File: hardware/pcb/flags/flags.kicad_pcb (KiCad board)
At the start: 2 copper layers, 62.2 x 21.6 mm, 42 parts, among them J1 Bus, J2 Control, J3 Sync, J4 Power, J5 Flags_Bus, J6 Ctrl_Out, U1 74HC02, U2 74HC08, U3 74HC157, U4 74HC173, U5 74HC173, U6 74HC125

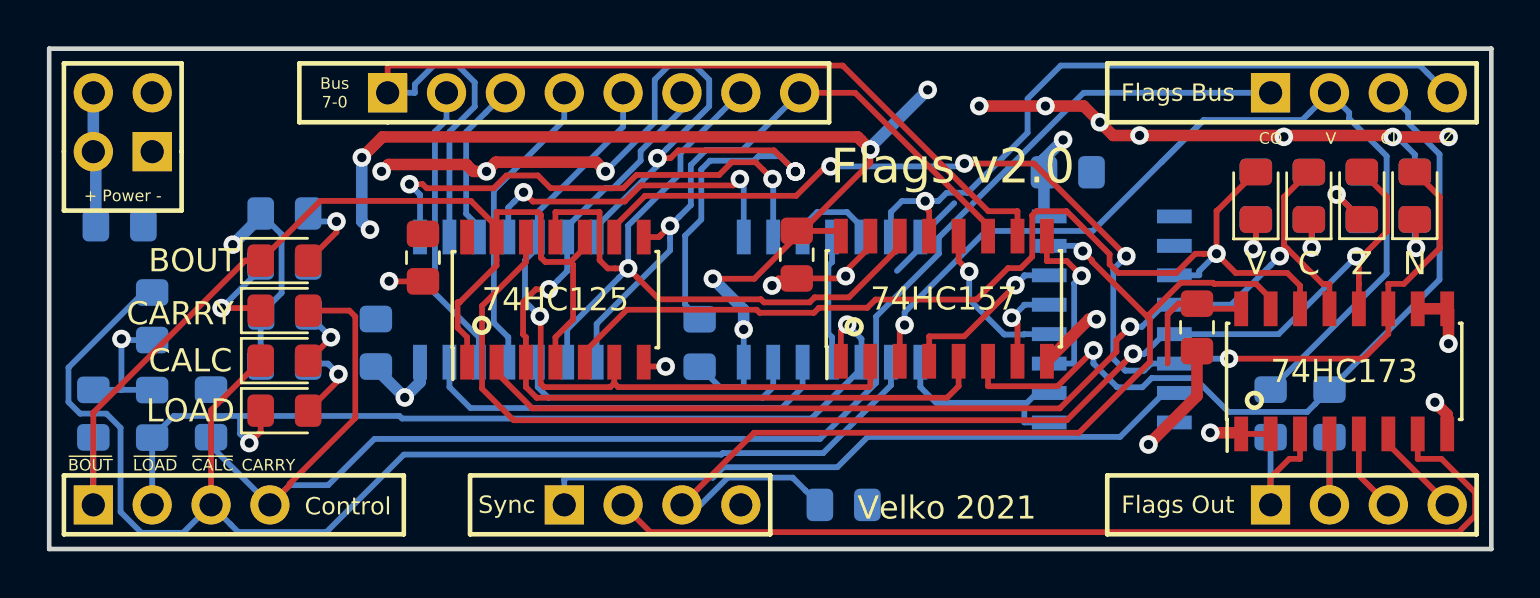
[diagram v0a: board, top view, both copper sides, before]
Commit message: Clean tracks again
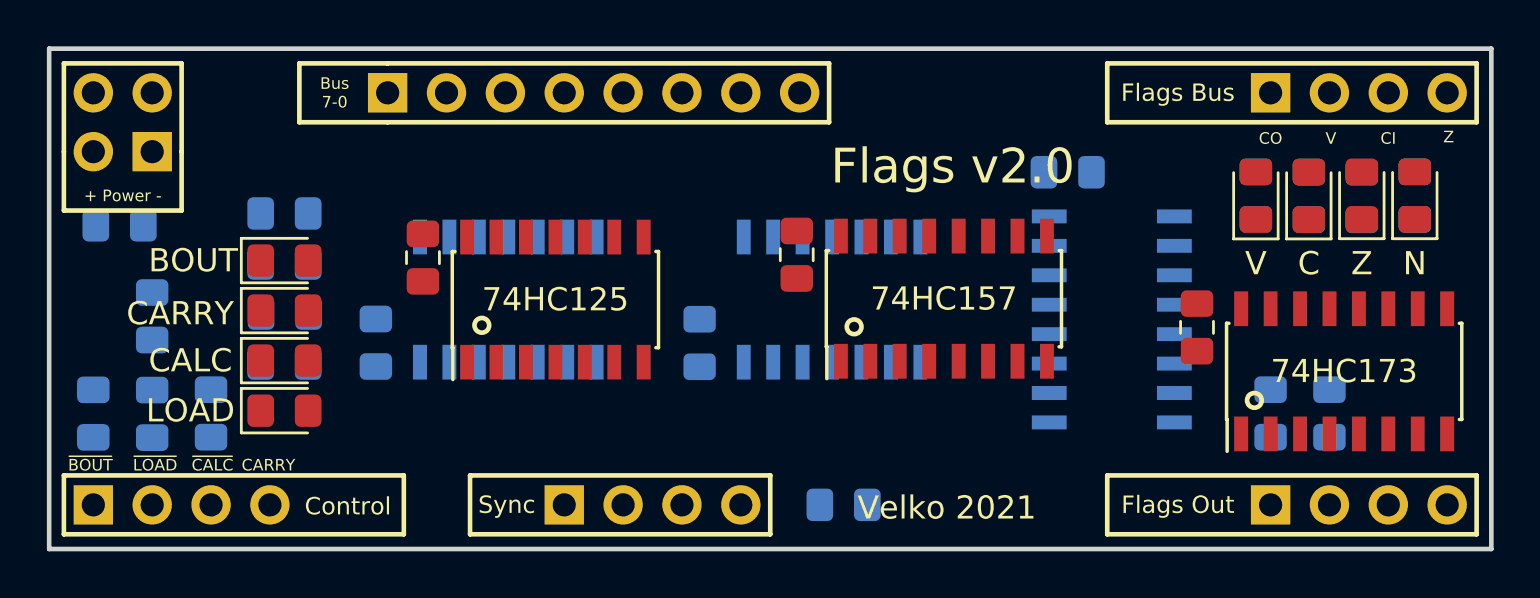
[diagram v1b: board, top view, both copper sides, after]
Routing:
- net GND: track 94.7 -> 0.00 mm, vias 22 -> 0
- net VCC: track 82.4 -> 0.00 mm, vias 10 -> 0
- net CARRY_OUT: track 68.4 -> 0.00 mm
- net ~B_CALC~: track 58.1 -> 0.00 mm
- net Z_D: track 55.6 -> 0.00 mm, vias 2 -> 0
- net N_D: track 51.3 -> 0.00 mm, vias 4 -> 0
- net ~OUT~: track 47.6 -> 0.00 mm
- net C_D: track 45.7 -> 0.00 mm, vias 2 -> 0
- net V_D: track 44.8 -> 0.00 mm, vias 1 -> 0
- net BUS7: track 43.9 -> 0.00 mm
- net RST: track 43.9 -> 0.00 mm, vias 1 -> 0
- net OV_IN: track 42.9 -> 0.00 mm, vias 1 -> 0
- net ~CLK~: track 42.7 -> 0.00 mm
- net ~B_LOAD~: track 41.6 -> 0.00 mm, vias 2 -> 0
- net BUS2: track 36.3 -> 0.00 mm, vias 1 -> 0
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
